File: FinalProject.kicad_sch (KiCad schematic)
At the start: 22 parts, among them U1 L78L05_TO92, U2 LM339

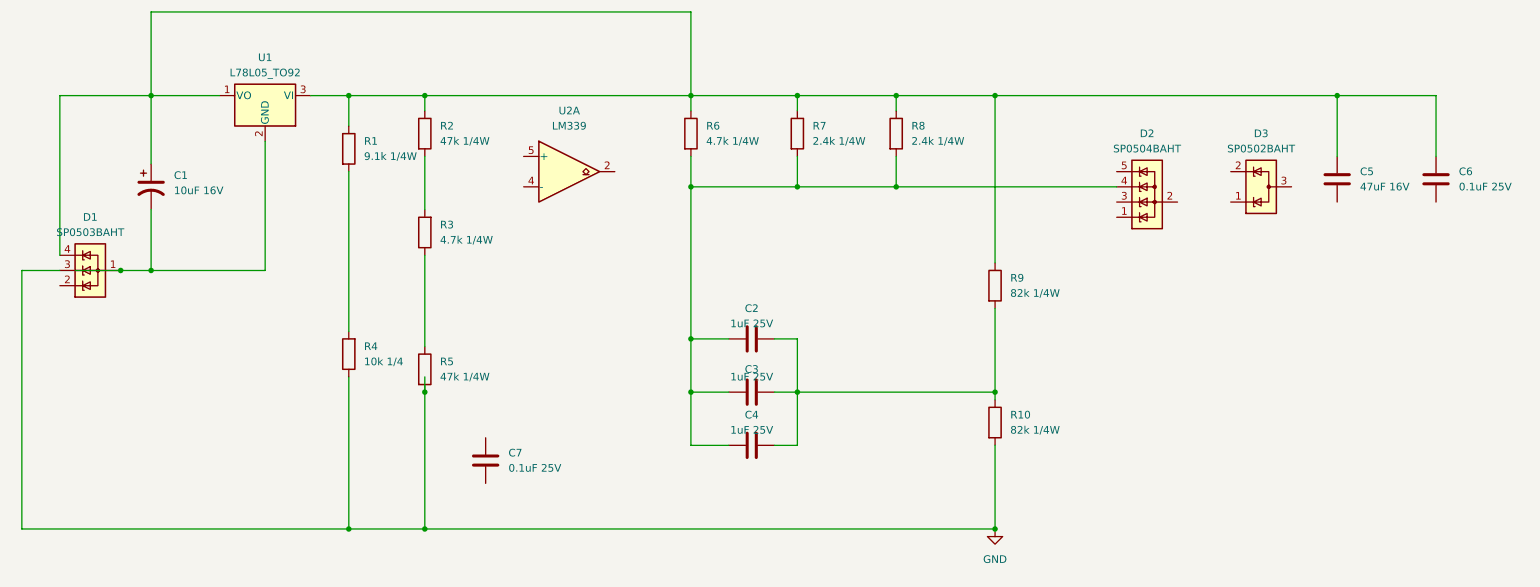
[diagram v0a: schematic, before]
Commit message: Add files via upload
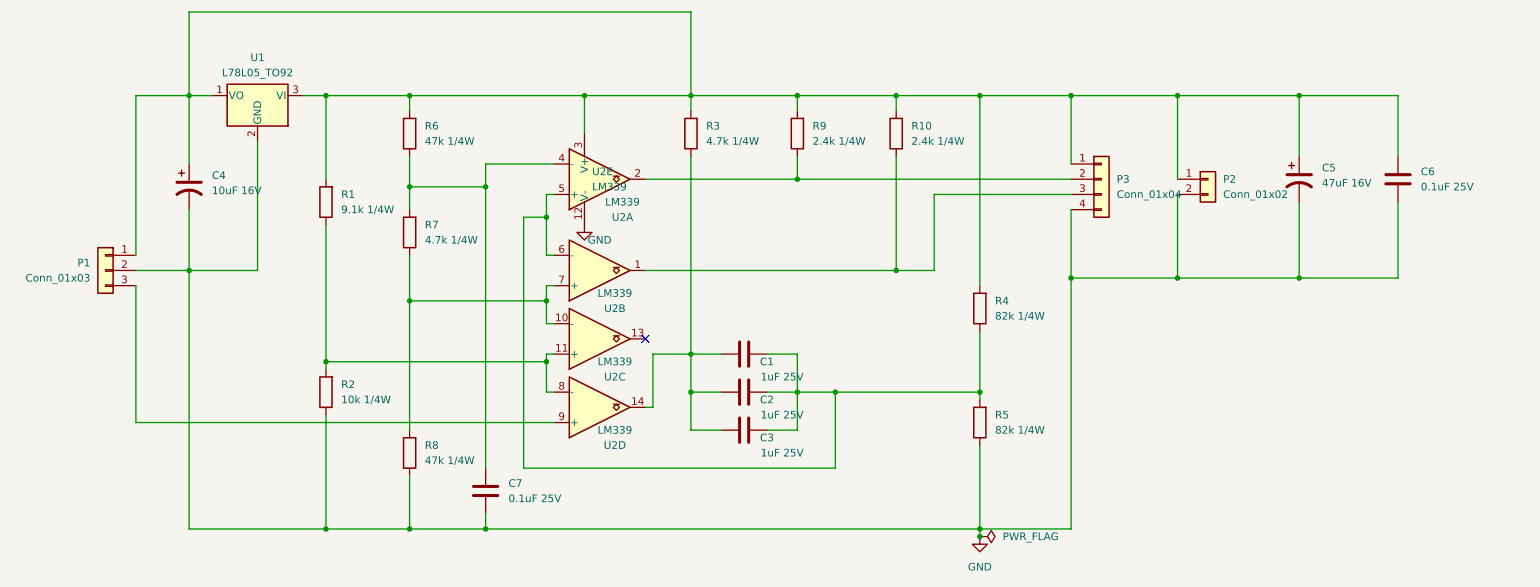
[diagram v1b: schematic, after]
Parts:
- removed C4: 1uF 25V, symbol Device:C
- removed C5: 47uF 16V, symbol Device:C
- removed D1: SP0503BAHT, Package_TO_SOT_SMD:SOT-143, symbol Power_Protection:SP0503BAHT
- removed D2: SP0504BAHT, Package_TO_SOT_SMD:SOT-353_SC-70-5, symbol Power_Protection:SP0504BAHT
- removed D3: SP0502BAHT, Package_TO_SOT_SMD:SOT-23, symbol Power_Protection:SP0502BAHT
- added C1: 1uF 25V, Capacitor_THT:C_Rect_L7.2mm_W3.5mm_P5.00mm_FKS2_FKP2_MKS2_MKP2, symbol Device:C
- added C5: 47uF 16V, Capacitor_THT:CP_Radial_D5.0mm_P2.50mm, symbol Device:C_Polarized_US
- added P1: Conn_01x03, Connector_PinHeader_2.54mm:PinHeader_1x03_P2.54mm_Vertical, symbol Connector_Generic:Conn_01x03
- added P2: Conn_01x02, Connector_Wire:SolderWire-0.5sqmm_1x02_P4.6mm_D0.9mm_OD2.1mm, symbol Connector_Generic:Conn_01x02
- added P3: Conn_01x04, Connector_PinHeader_2.54mm:PinHeader_1x04_P2.54mm_Vertical, symbol Connector_Generic:Conn_01x04
- added unit 3 of U2
- added unit 2 of U2
- added unit 4 of U2
- added unit 5 of U2
- C2, C3: footprint (none) -> Capacitor_THT:C_Rect_L7.2mm_W3.5mm_P5.00mm_FKS2_FKP2_MKS2_MKP2
- C4: renamed from C1; footprint (none) -> Capacitor_THT:CP_Radial_D5.0mm_P2.50mm
- C6, C7: footprint (none) -> Capacitor_THT:C_Rect_L7.2mm_W3.0mm_P5.00mm_FKS2_FKP2_MKS2_MKP2
- R1, R3: footprint (none) -> Resistor_THT:R_Axial_DIN0207_L6.3mm_D2.5mm_P10.16mm_Horizontal
- R10, R9: value 82k 1/4W -> 2.4k 1/4W; footprint (none) -> Resistor_THT:R_Axial_DIN0207_L6.3mm_D2.5mm_P10.16mm_Horizontal
- R2: value 47k 1/4W -> 10k 1/4W; footprint (none) -> Resistor_THT:R_Axial_DIN0207_L6.3mm_D2.5mm_P10.16mm_Horizontal
- R4: value 10k 1/4 -> 82k 1/4W; footprint (none) -> Resistor_THT:R_Axial_DIN0207_L6.3mm_D2.5mm_P10.16mm_Horizontal
- R5: value 47k 1/4W -> 82k 1/4W; footprint (none) -> Resistor_THT:R_Axial_DIN0207_L6.3mm_D2.5mm_P10.16mm_Horizontal
- R6: value 4.7k 1/4W -> 47k 1/4W; footprint (none) -> Resistor_THT:R_Axial_DIN0207_L6.3mm_D2.5mm_P10.16mm_Horizontal
- R7: value 2.4k 1/4W -> 4.7k 1/4W; footprint (none) -> Resistor_THT:R_Axial_DIN0207_L6.3mm_D2.5mm_P10.16mm_Horizontal
- R8: value 2.4k 1/4W -> 47k 1/4W; footprint (none) -> Resistor_THT:R_Axial_DIN0207_L6.3mm_D2.5mm_P10.16mm_Horizontal
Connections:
- net GND: now also C4.2, C6.2, C7.2, R2.1, R5.1, R8.1, U1.2 (GND), C5.2, P1.2 (Pin_2), P2.2 (Pin_2), P3.4 (Pin_4), U2.12 (V-); no longer R10.2, R4.1, R5.2
- net at R1.2, R4.2: now also C4.1, C6.1, R10.2, R3.2, R6.2, R9.2, U1.1 (VO), U1.3 (VI), C5.1, P1.1 (Pin_1), P2.1 (Pin_1), P3.1 (Pin_1), U2.3 (V+)
- net at C2.2, C3.2: now also R4.1, R5.2, U2.5 (+), C1.2, U2.6 (-); no longer R10.1, R9.2
- net at C7.1: now also R6.1, R7.2, U2.4 (-)
- net at R3.1: now also C2.1, C3.1, C1.1, U2.14; no longer R5.1
- net at R2.2: now also R1.1, U2.11 (+), U2.8 (-); no longer R3.2
- net at U2.2: now also R9.1, P3.2 (Pin_2)
- new net: R7.1, R8.2, U2.10 (-), U2.7 (+)
- new net: P3.3 (Pin_3), R10.1, U2.1
- new net: P1.3 (Pin_3), U2.9 (+)
- no-connect marks 0 -> 1
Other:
- moved on the sheet: C4, C7, U2A
